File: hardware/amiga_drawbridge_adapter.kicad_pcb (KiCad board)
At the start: 2 copper layers, 44.4 x 49.5 mm, 18 parts, among them J1 FTDI_232_RED, J2 DiskDrive Power, J3 PC3-PC5, J4 AVR-ISP-6, J5 DiskDrive Data, SW1 SW_Push, U1 ATmega328P-A, Y1 16MHz

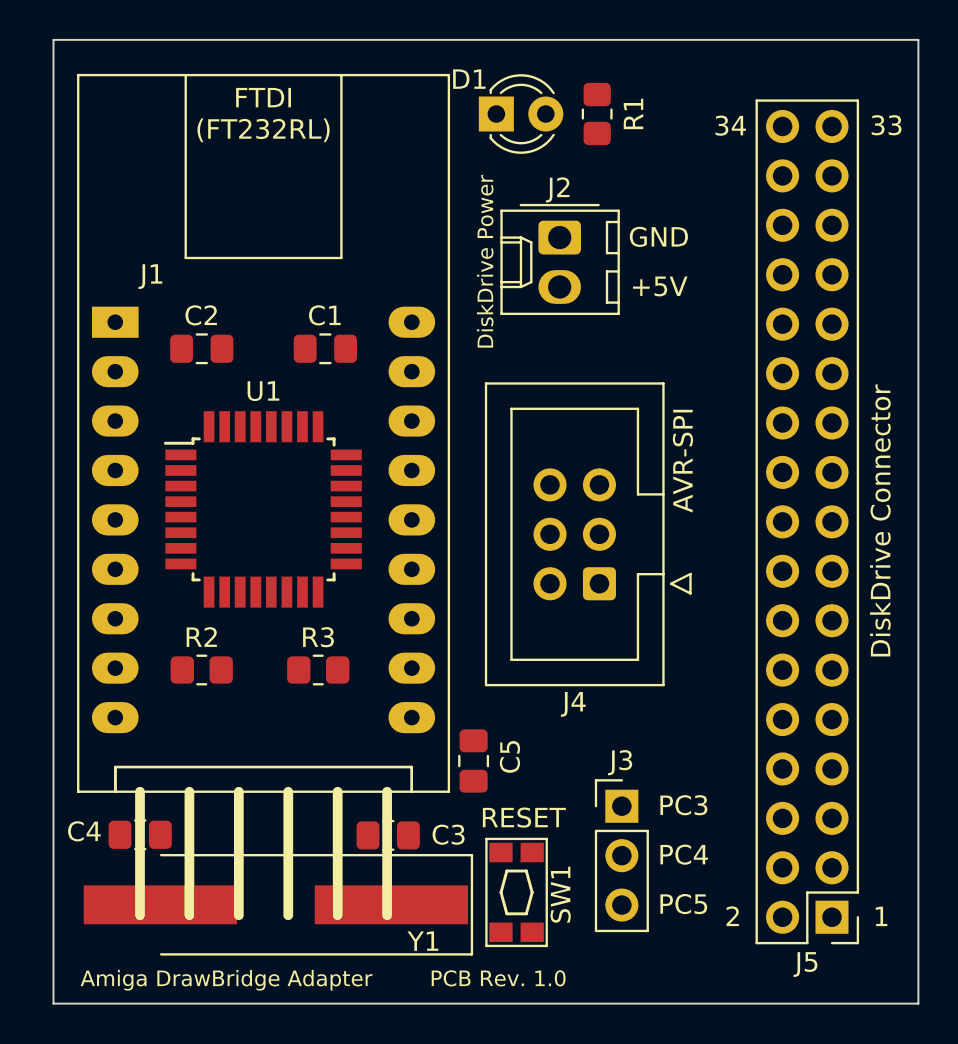
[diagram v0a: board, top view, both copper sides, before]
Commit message: added pictures and routing pcb
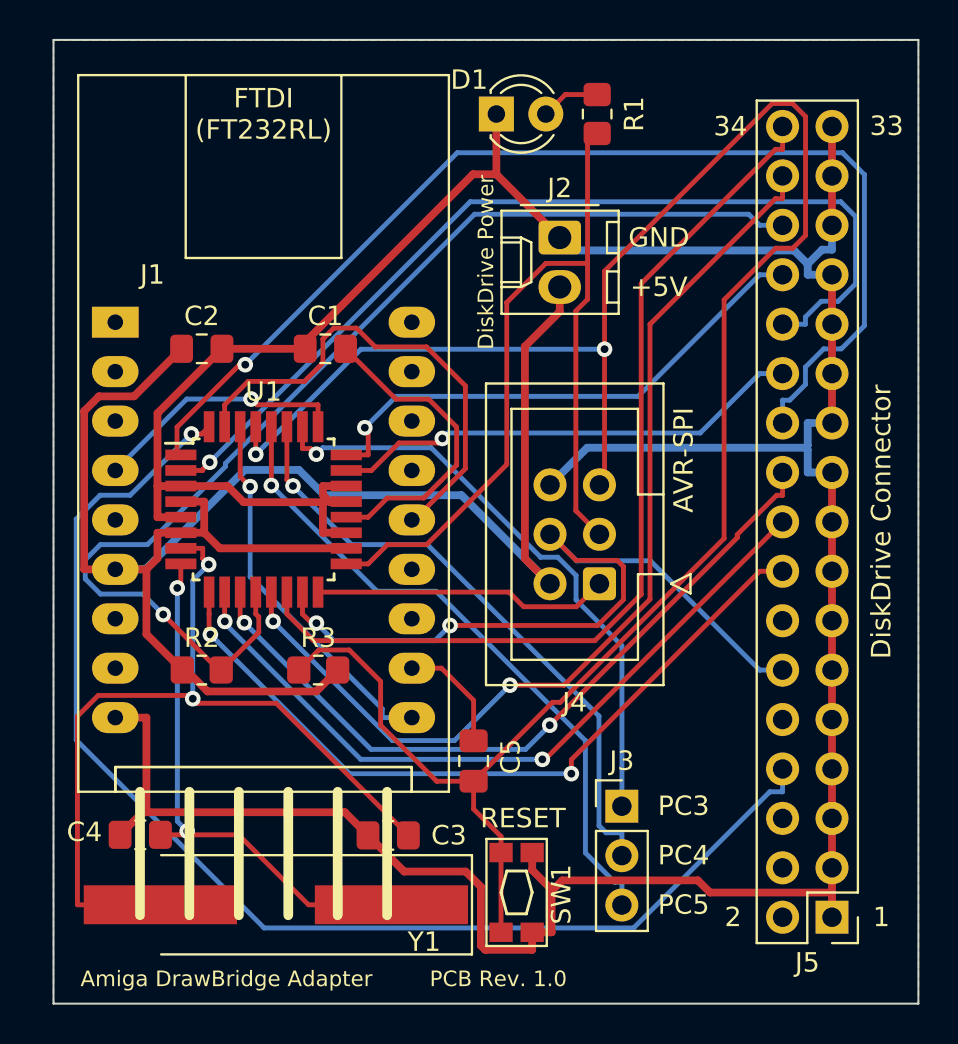
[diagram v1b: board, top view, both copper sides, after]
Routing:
- net GND: track 0.00 -> 178.6 mm
- net RESET: track 0.00 -> 110.7 mm, vias 0 -> 2
- net VCC: track 0.00 -> 90.9 mm
- net DRV_INDEX: track 0.00 -> 64.5 mm, vias 0 -> 1
- net DRV_WRITE_DATA: track 0.00 -> 58.4 mm, vias 0 -> 1
- net DRV_READ_DATA: track 0.00 -> 58.3 mm, vias 0 -> 1
- net DRV_HEAD_SELECT: track 0.00 -> 51.3 mm, vias 0 -> 2
- net DRV_TRACK_0: track 0.00 -> 49.0 mm, vias 0 -> 1
- net DRV_DISK_CHANGE: track 0.00 -> 48.2 mm
- net LED: track 0.00 -> 45.2 mm
- net Net-(C3-Pad1): track 0.00 -> 43.7 mm, vias 0 -> 2
- net DRV_SEL_B: track 0.00 -> 40.1 mm, vias 0 -> 2
- net DRV_MOTOR_EN_B: track 0.00 -> 39.3 mm, vias 0 -> 2
- net DRV_STEP: track 0.00 -> 38.7 mm, vias 0 -> 2
- net DRV_DIRECTION: track 0.00 -> 38.2 mm, vias 0 -> 2
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- added copper zone on B.Cu, net GND
- added copper zone on F.Cu, net GND

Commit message: create gerberfiles rev1.0
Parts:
- R1: value 82 -> 100
